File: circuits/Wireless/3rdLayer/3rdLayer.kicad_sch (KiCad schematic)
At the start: 9 parts, among them J1 USB_C_Receptacle_USB2.0, U1 CH340E

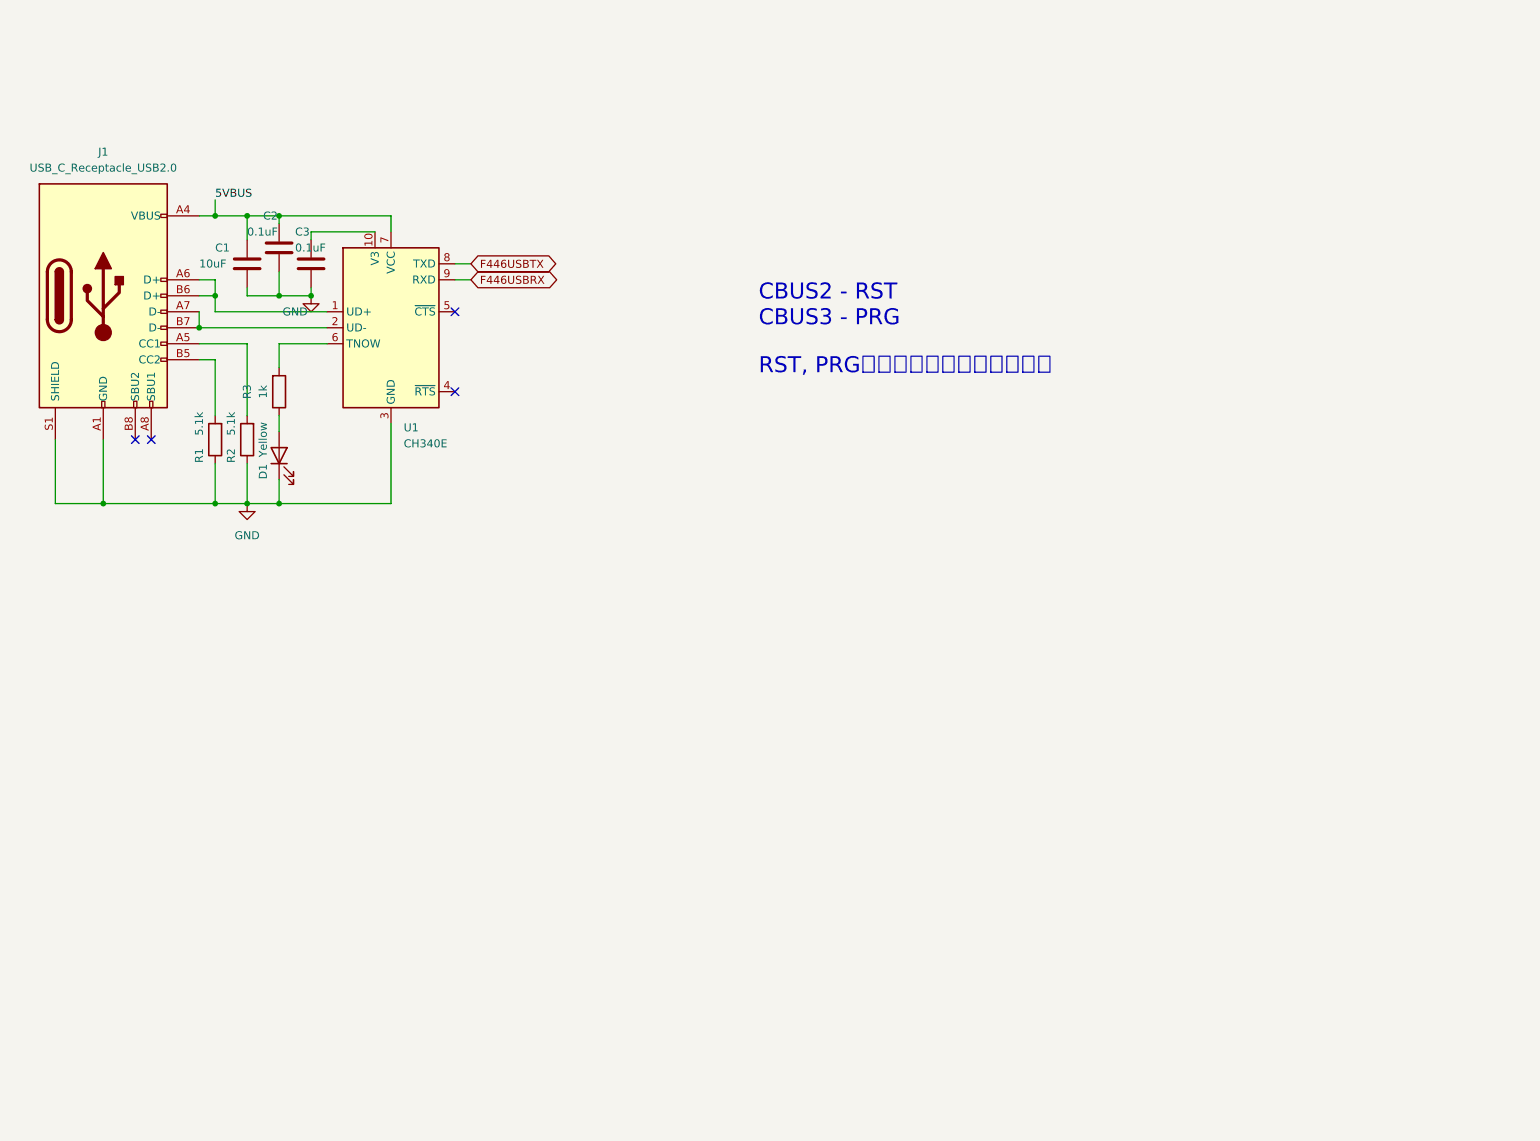
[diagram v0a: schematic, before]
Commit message: 無線&UI完成？
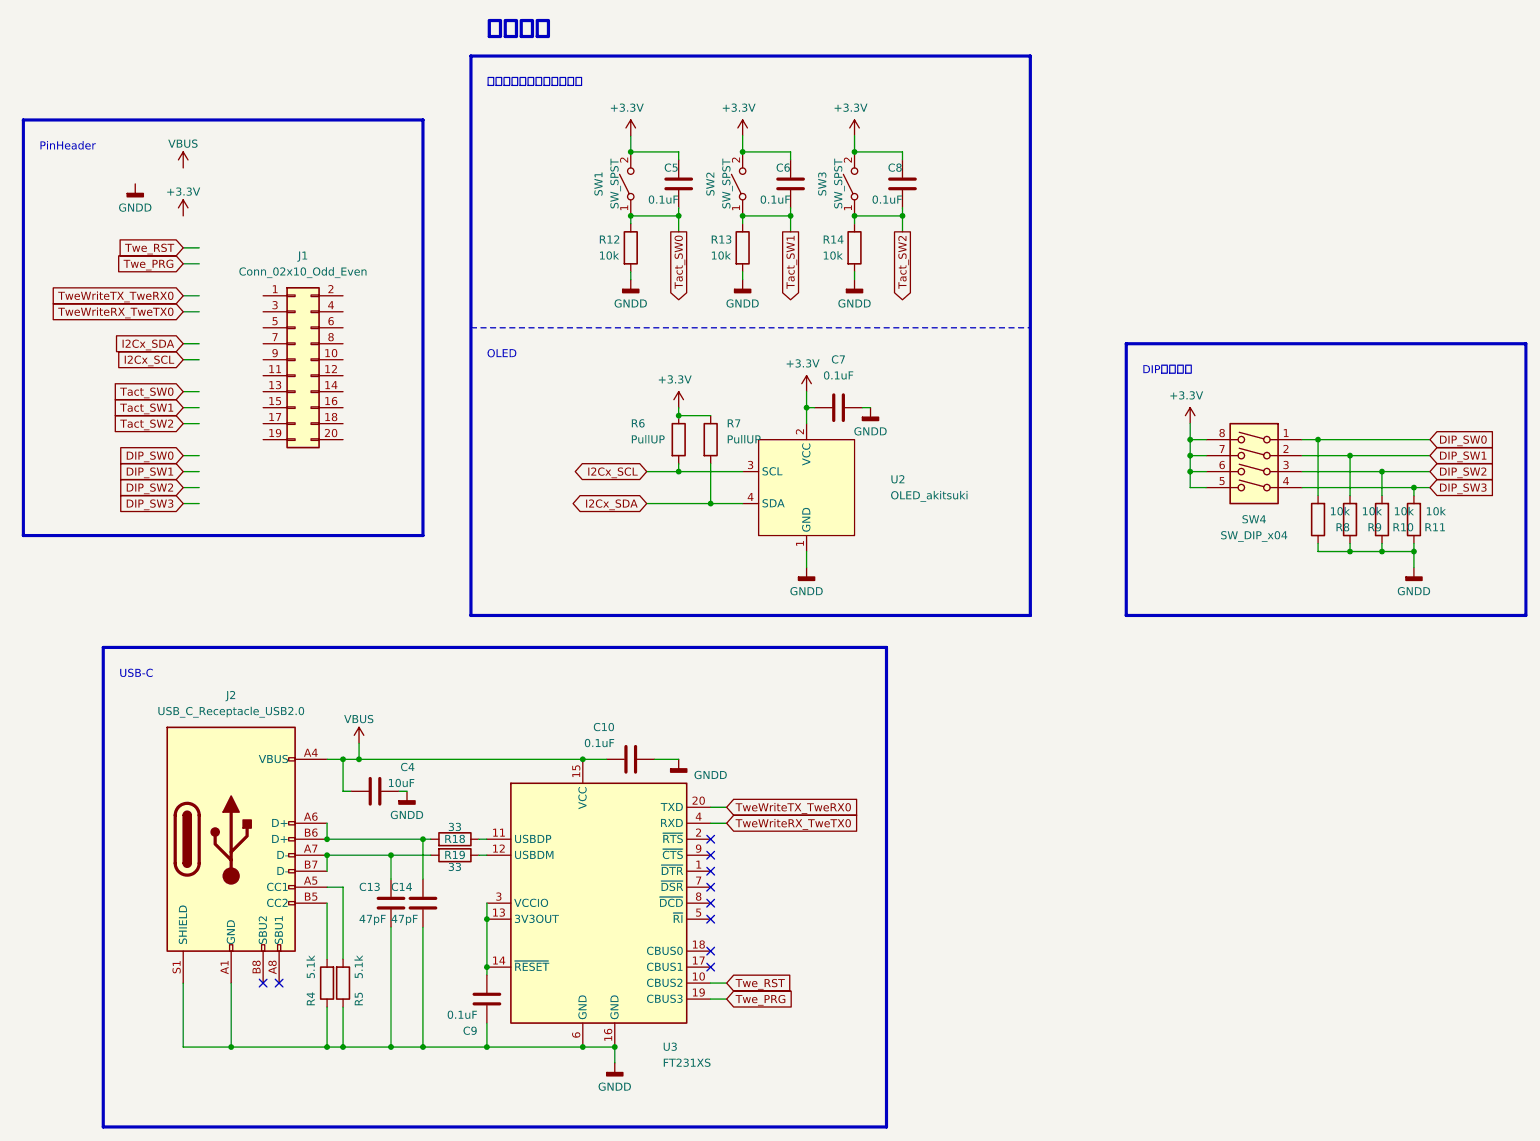
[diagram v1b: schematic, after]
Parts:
- removed C1: 10uF, Capacitor_SMD:C_0805_2012Metric, symbol Device:C
- removed C2, C3: 0.1uF, Capacitor_SMD:C_0402_1005Metric, symbol Device:C
- removed D1: Yellow, LED_SMD:LED_0603_1608Metric_Pad1.05x0.95mm_HandSolder, symbol Device:LED
- removed J1: USB_C_Receptacle_USB2.0, Connector_USB:USB_C_Receptacle_G-Switch_GT-USB-7010ASV, symbol Connector:USB_C_Receptacle_USB2.0
- removed R1, R2: 5.1k, Resistor_SMD:R_0402_1005Metric, symbol Device:R
- removed R3: 1k, Resistor_SMD:R_0402_1005Metric, symbol Device:R
- removed U1: CH340E, Package_SO:MSOP-10_3x3mm_P0.5mm, symbol Interface_USB:CH340E
- added C10, C5, C6, C7, C8, C9: 0.1uF, Capacitor_SMD:C_0402_1005Metric, symbol Device:C
- added C13, C14: 47pF, Capacitor_SMD:C_0603_1608Metric, symbol Device:C
- added C4: 10uF, Capacitor_SMD:C_0805_2012Metric, symbol Device:C
- added J1: Conn_02x10_Odd_Even, Connector_PinHeader_1.27mm:PinHeader_2x10_P1.27mm_Vertical, symbol Connector_Generic:Conn_02x10_Odd_Even
- added J2: USB_C_Receptacle_USB2.0, Connector_USB:USB_C_Receptacle_G-Switch_GT-USB-7010ASV, symbol Connector:USB_C_Receptacle_USB2.0
- added R10, R11, R12, R13, R14, R8, R9: 10k, Resistor_SMD:R_0402_1005Metric, symbol Device:R
- added R18, R19: 33, Resistor_SMD:R_0603_1608Metric, symbol Device:R
- added R4, R5: 5.1k, Resistor_SMD:R_0402_1005Metric, symbol Device:R
- added R6, R7: PullUP, Resistor_SMD:R_0603_1608Metric_Pad0.98x0.95mm_HandSolder, symbol Device:R
- added SW1, SW2, SW3: SW_SPST, Button_Switch_SMD:SW_SPST_Omron_B3FS-100xP, symbol Switch:SW_SPST
- added SW4: SW_DIP_x04, Button_Switch_SMD:SW_DIP_SPSTx04_Slide_Copal_CHS-04B_W7.62mm_P1.27mm, symbol Switch:SW_DIP_x04
- added U2: OLED_akitsuki, Display_akitsuki:128×64_OLED_White, symbol Display:OLED_akitsuki
- added U3: FT231XS, Package_SO:SSOP-20_3.9x8.7mm_P0.635mm, symbol Interface_USB:FT231XS
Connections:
- new net: R19.1, U3.12 (USBDM)
- new net: C13.1, J2.A7 (D-), J2.B7 (D-), R19.2
- new net: C9.2, U3.13 (3V3OUT), U3.14 (~{RESET}), U3.3 (VCCIO)
- new net: R18.1, U3.11 (USBDP)
- new net: C14.1, J2.A6 (D+), J2.B6 (D+), R18.2
- new net: J2.A5 (CC1), R5.2
- new net: J2.B5 (CC2), R4.2
- new net +3.3V: C5.1, C6.1, C7.1, C8.1, R6.1, R7.1, SW1.2 (B), SW2.2 (B), SW3.2 (B), SW4.5, SW4.6, SW4.7, SW4.8, U2.2 (VCC)
- new net DIP_SW0: R8.2, SW4.1
- new net DIP_SW1: R9.2, SW4.2
- new net DIP_SW2: R10.2, SW4.3
- new net DIP_SW3: R11.2, SW4.4
- new net GNDD: C10.2, C13.2, C14.2, C4.1, C7.2, C9.1, J2.A1 (GND), J2.A12 (GND), J2.B1 (GND), J2.B12 (GND), J2.S1 (SHIELD), R10.1, R11.1, R12.2, R13.2, R14.2, R4.1, R5.1, R8.1, R9.1, U2.1 (GND), U3.16 (GND), U3.6 (GND)
- new net I2Cx_SCL: R6.2, U2.3 (SCL)
- new net I2Cx_SDA: R7.2, U2.4 (SDA)
- new net Tact_SW0: C5.2, R12.1, SW1.1 (A)
- new net Tact_SW1: C6.2, R13.1, SW2.1 (A)
- new net Tact_SW2: C8.2, R14.1, SW3.1 (A)
- new net TweWriteRX_TweTX0: U3.4 (RXD)
- new net TweWriteTX_TweRX0: U3.20 (TXD)
- new net Twe_PRG: U3.19 (CBUS3)
- new net Twe_RST: U3.10 (CBUS2)
- new net VBUS: C10.1, C4.2, J2.A4 (VBUS), J2.A9 (VBUS), J2.B4 (VBUS), J2.B9 (VBUS), U3.15 (VCC)
- no-connect marks 4 -> 10
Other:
- note added: "DIPスイッチ"
- note added: "OLED"
- note added: "PinHeader"
- note added: "USB-C"
- note added: "モニター"
- note added: "モニター用タクトスイッチ"
- note removed: "CBUS2 - RST CBUS3 - PRG"
- note removed: "RST, PRGどっちもプルアップ付ける"
